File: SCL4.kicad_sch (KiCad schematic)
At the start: 4 parts

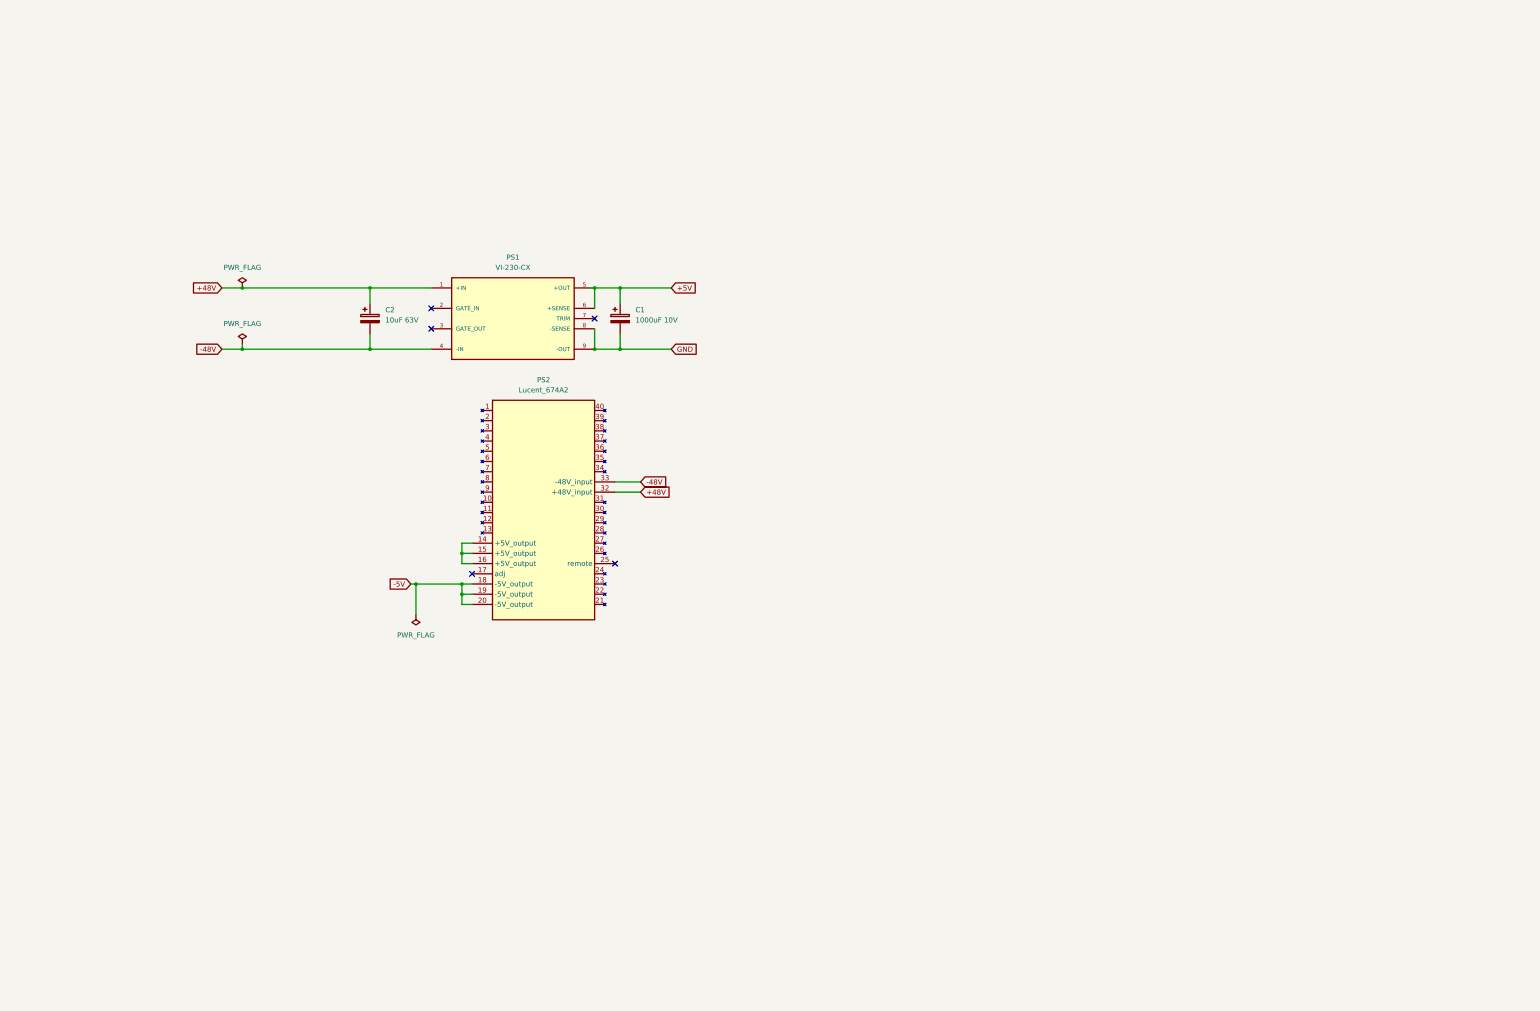
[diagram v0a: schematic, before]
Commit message: ERC passes
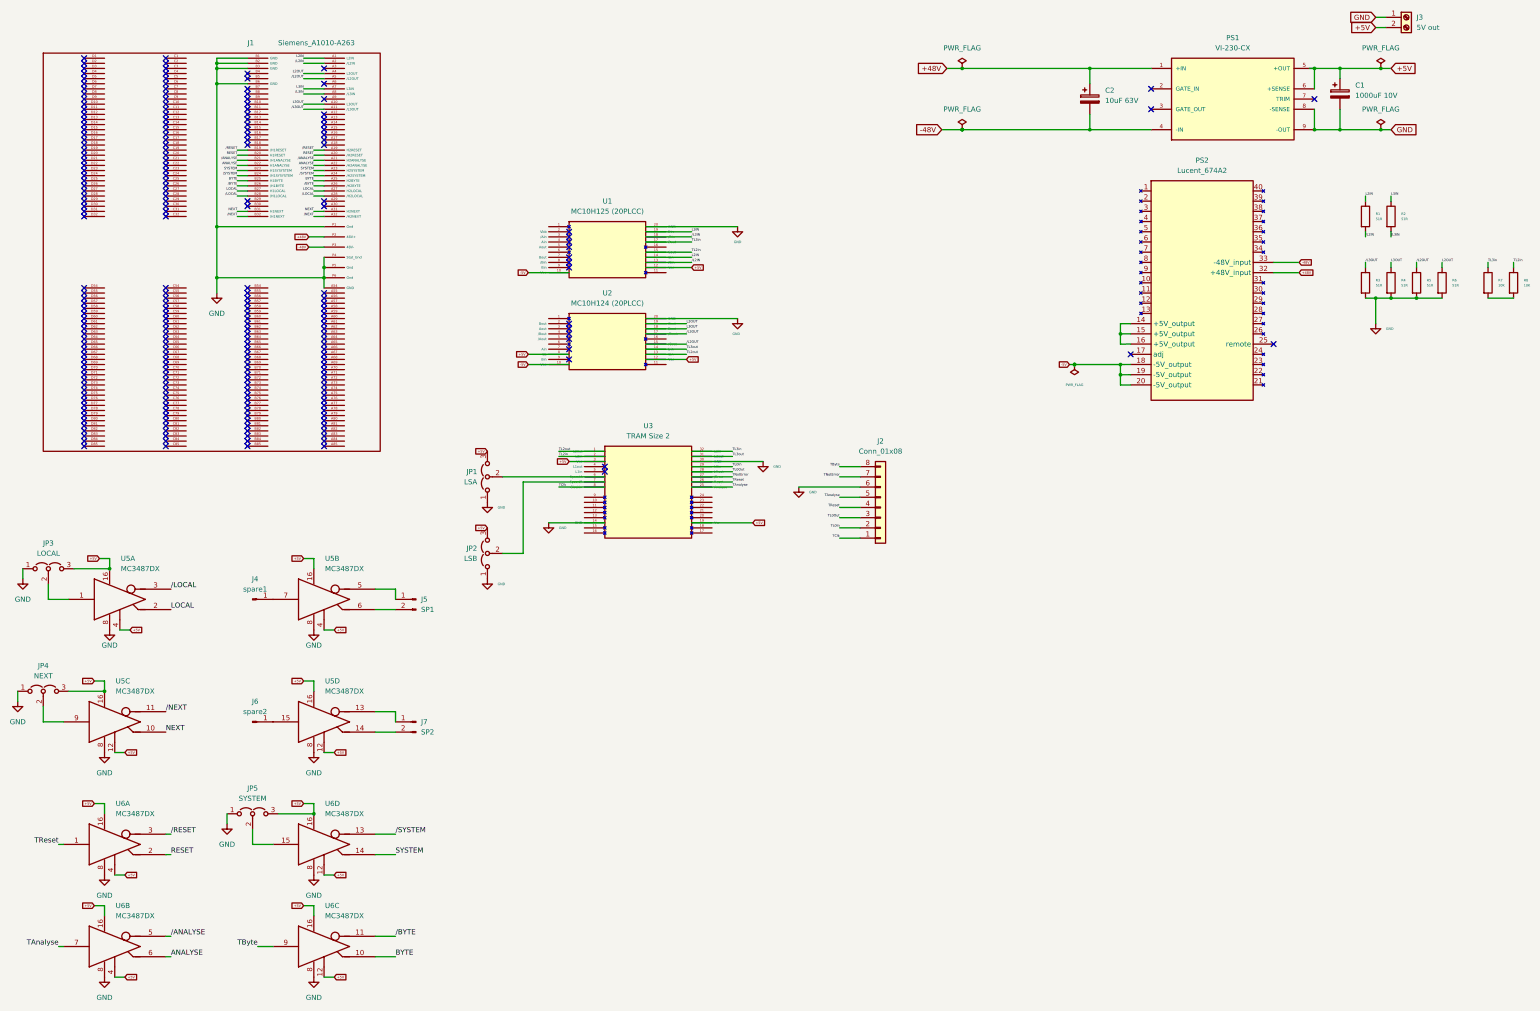
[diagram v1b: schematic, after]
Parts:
- added J1: Siemens_A1010-A263, symbol siemens_a1010-a263:Siemens_A1010-A263
- added J2: Conn_01x08, symbol Connector_Generic:Conn_01x08
- added J3: 5V out, symbol Connector:Screw_Terminal_01x02
- added J4: spare1, symbol Connector:Conn_01x01_Male
- added J5: SP1, symbol Connector:Conn_01x02_Male
- added J6: spare2, symbol Connector:Conn_01x01_Male
- added J7: SP2, symbol Connector:Conn_01x02_Male
- added JP1: LSA, symbol Jumper:Jumper_3_Open
- added JP2: LSB, symbol Jumper:Jumper_3_Open
- added JP3: LOCAL, symbol Jumper:Jumper_3_Open
- added JP4: NEXT, symbol Jumper:Jumper_3_Open
- added JP5: SYSTEM, symbol Jumper:Jumper_3_Open
- added R1, R2, R3, R4, R5, R6: 51R, symbol Device:R
- added R7, R8: 10K, symbol Device:R
- added U1: MC10H125 (20PLCC), symbol Interface:MC10H125 (20PLCC)
- added U2: MC10H124 (20PLCC), symbol Interface:MC10H124 (20PLCC)
- added U3: TRAM Size 2, symbol Transputer:TRAM Size 2
- added U5, U6: MC3487DX, Package_SO:SOIC-16_3.9x9.9mm_P1.27mm, symbol Interface_LineDriver:MC3487DX
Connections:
- net +48V: now also J1.P2 (48V+)
- net +5V: now also J3.2 (Pin_2), JP1.3 (B), JP2.3 (B), JP3.3 (B), JP4.3 (B), JP5.3 (B), U1.12 (Vcc), U2.12 (Vcc), U2.8 (CS), U3.19 (Vcc), U3.3 (Vcc), U5.12 (ENABLE), U5.12 (ENABLE), U5.16 (VCC), U5.16 (VCC), U5.16 (VCC), U5.16 (VCC), U5.4 (ENABLE), U5.4 (ENABLE), U6.12 (ENABLE), U6.12 (ENABLE), U6.16 (VCC), U6.16 (VCC), U6.16 (VCC), U6.16 (VCC), U6.4 (ENABLE), U6.4 (ENABLE)
- net -48V: now also J1.P3 (48V-)
- net -5V: now also U1.10 (Vee), U2.10 (Vee)
- net GND: now also J1.A54 (GND), J1.B1 (GND), J1.B2 (GND), J1.B3 (GND), J1.B6 (GND), J1.P1 (Gnd), J1.P4 (Stat_Gnd), J1.P5 (Gnd), J1.P6 (Gnd), J2.6 (Pin_6), J3.1 (Pin_1), JP1.1 (A), JP2.1 (A), JP3.1 (A), JP4.1 (A), JP5.1 (A), R3.2, R4.2, R5.2, R6.2, U1.20 (GND), U2.20 (GND), U3.14 (GND), U3.30 (GND), U5.8 (GND), U5.8 (GND), U5.8 (GND), U5.8 (GND), U6.8 (GND), U6.8 (GND), U6.8 (GND), U6.8 (GND)
- new net: JP1.2 (C), U3.6 (SpeedA)
- new net: JP4.2 (C), U5.9 (INPUT)
- new net: JP3.2 (C), U5.1 (INPUT)
- new net: JP2.2 (C), U3.7 (SpeedB)
- new net: J7.1 (Pin_1), U5.13 (OUT-)
- new net: J7.2 (Pin_2), U5.14 (OUT+)
- new net: R7.2, R8.2
- new net: JP5.2 (C), U6.15 (INPUT)
- new net: J6.1 (Pin_1), U5.15 (INPUT)
- new net: J5.1 (Pin_1), U5.5 (OUT-)
- new net: J5.2 (Pin_2), U5.6 (OUT+)
- new net: J4.1 (Pin_1), U5.7 (INPUT)
- new net ANALYSE: J1.A22 (/H2ANALYSE), J1.B22 (H1ANALYSE), U6.6 (OUT+)
- new net BYTE: J1.A25 (H2BYTE), J1.B25 (H1BYTE), U6.10 (OUT+)
- new net L2IN: J1.A1 (L2IN), R1.1, U1.14 (Cin)
- new net L2OUT: J1.A4 (L2OUT), R6.1, U2.19 (Cout)
- new net L3IN: J1.A7 (L3IN), R2.1, U1.19 (Din)
- new net L3OUT: J1.A10 (L3OUT), R4.1, U2.18 (Dout)
- new net LOCAL: J1.A27 (H2LOCAL), J1.B27 (H1LOCAL), U5.2 (OUT+)
- new net NEXT: J1.A31 (H2NEXT), J1.B31 (H1NEXT), U5.10 (OUT+)
- new net RESET: J1.A20 (/H2RESET), J1.B20 (H1RESET), U6.2 (OUT+)
- new net SYSTEM: J1.A23 (H2SYSTEM), J1.B23 (H1SYSYSTEM), U6.14 (OUT+)
- new net TAnalyse: J2.5 (Pin_5), U3.25 (Analyse), U6.7 (INPUT)
- new net TByte: J2.8 (Pin_8), U6.9 (INPUT)
- new net TClk: J2.1 (Pin_1), U3.8 (ClockIn)
- new net TL0In: J2.2 (Pin_2), U3.29 (L0in)
- new net TL0Out: J2.3 (Pin_3), U3.28 (L0out)
- new net TL2in: R8.1, U1.15 (Cout), U3.2 (L2in)
- new net TL2out: U2.13 (Cin), U3.1 (L2out)
- new net TL3in: R7.1, U1.17 (Dout), U3.32 (L3in)
- new net TL3out: U2.14 (Din), U3.31 (L3out)
- new net TNotError: J2.7 (Pin_7), U3.27 (/Error)
- new net TReset: J2.4 (Pin_4), U3.26 (Reset), U6.1 (INPUT)
- new net /ANALYSE: J1.A21 (H2ANALYSE), J1.B21 (/H1ANALYSE), U6.5 (OUT-)
- new net /BYTE: J1.A26 (/H2BYTE), J1.B26 (/H1BYTE), U6.11 (OUT-)
- new net /L2IN: J1.A2 (/L2IN), R1.2, U1.13 (/Cin)
- new net /L2OUT: J1.A5 (/L2OUT), R5.1, U2.15 (/Cout)
- new net /L3IN: J1.A8 (/L3IN), R2.2, U1.18 (/Din)
- new net /L3OUT: J1.A11 (/L3OUT), R3.1, U2.17 (/Dout)
- new net /LOCAL: J1.A28 (/H2LOCAL), J1.B28 (/H1LOCAL), U5.3 (OUT-)
- new net /NEXT: J1.A32 (/H2NEXT), J1.B32 (/H1NEXT), U5.11 (OUT-)
- new net /RESET: J1.A19 (H2RESET), J1.B19 (/H1RESET), U6.3 (OUT-)
- new net /SYSTEM: J1.A24 (/H2SYSTEM), J1.B24 (/H1SYSYSTEM), U6.13 (OUT-)
- no-connect marks 5 -> 239
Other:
- moved on the sheet: C1, C2, PS1, PS2
